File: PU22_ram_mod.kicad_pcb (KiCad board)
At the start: 2 copper layers, 39.1 x 104.6 mm, 11 parts, among them J1 MOBO, J2 BA8, J3 BA10

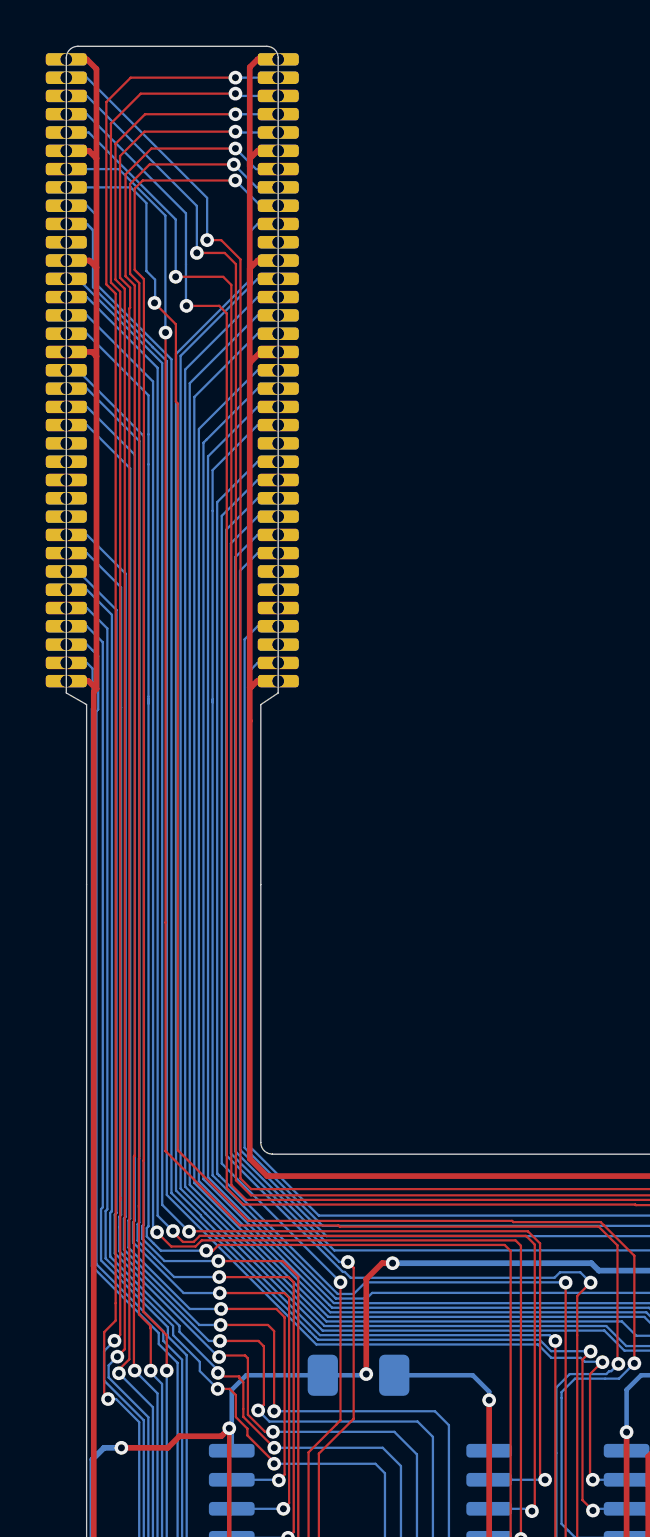
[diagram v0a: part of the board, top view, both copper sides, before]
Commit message: More routing
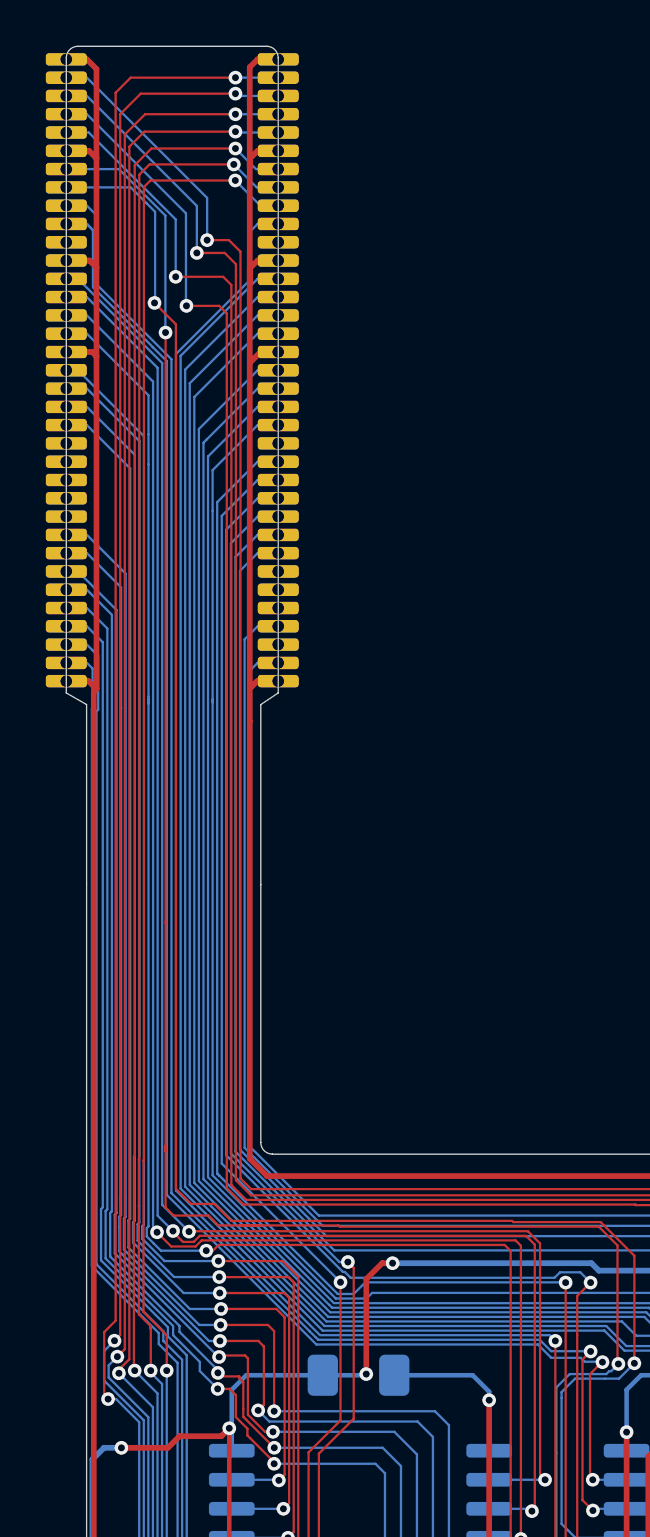
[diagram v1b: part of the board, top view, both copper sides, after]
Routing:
- net /D4: track 86.7 -> 89.2 mm
- net /D5: track 85.0 -> 86.0 mm
- net /D25: track 100.7 -> 100.2 mm
